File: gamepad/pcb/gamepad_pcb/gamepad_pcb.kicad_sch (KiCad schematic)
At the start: 9 parts, among them J1 RP CON R, J2 RP CON L, J3 JOYSTICK, SW1 BTN MINUS, SW2 BTN PLUS, SW3 BTN NORTH, SW4 BTN EAST, SW5 BTN SOUTH, SW6 BTN WEST

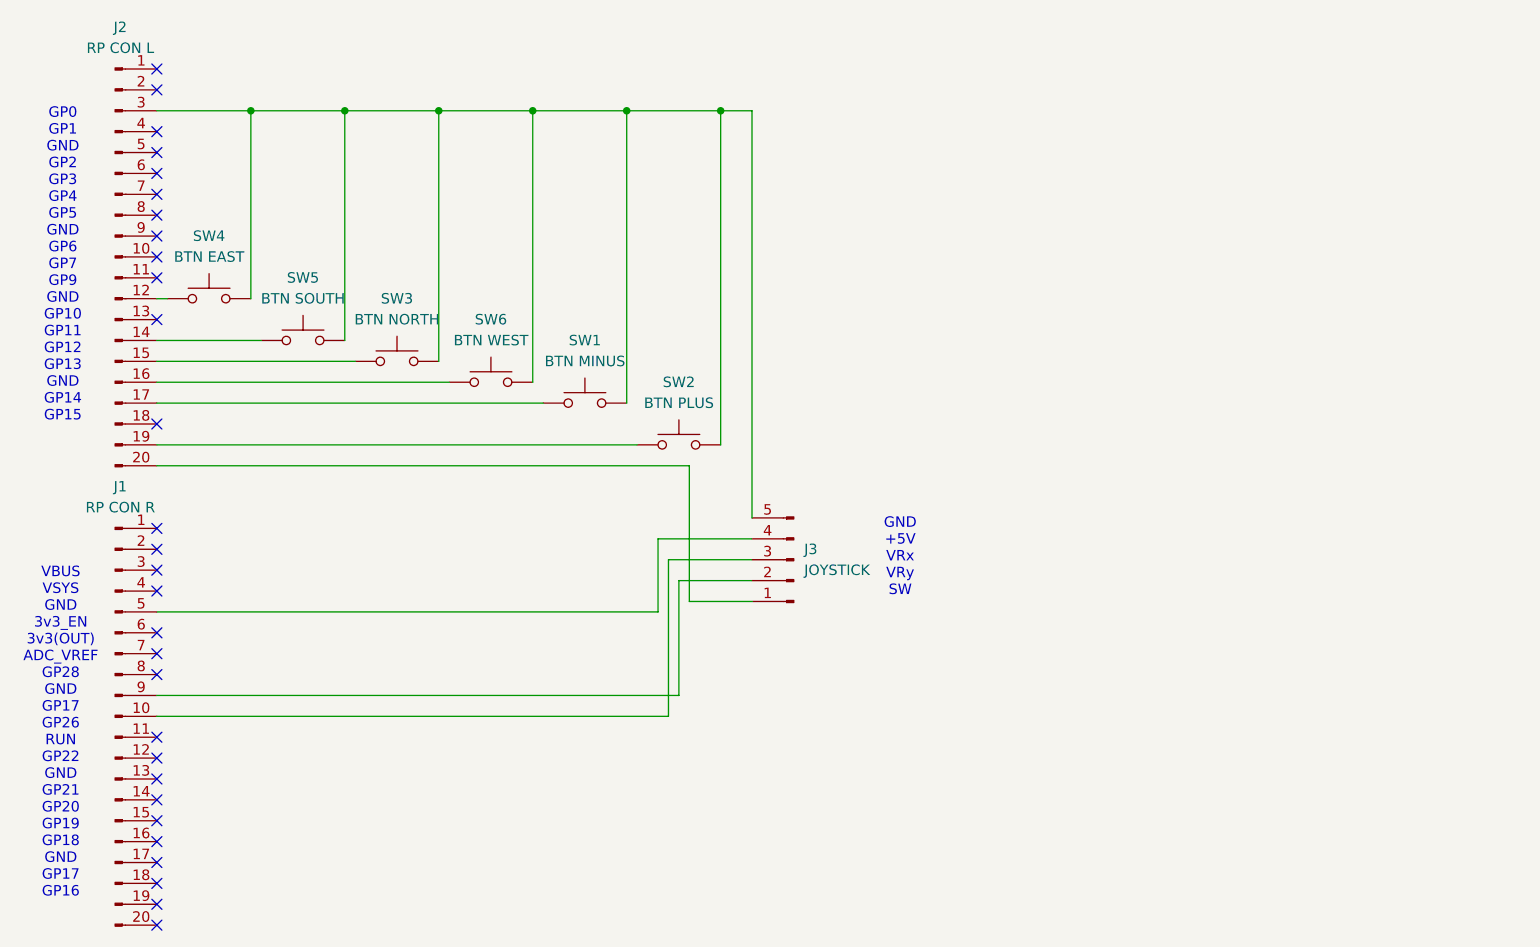
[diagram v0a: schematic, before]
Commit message: feat: working on pcb
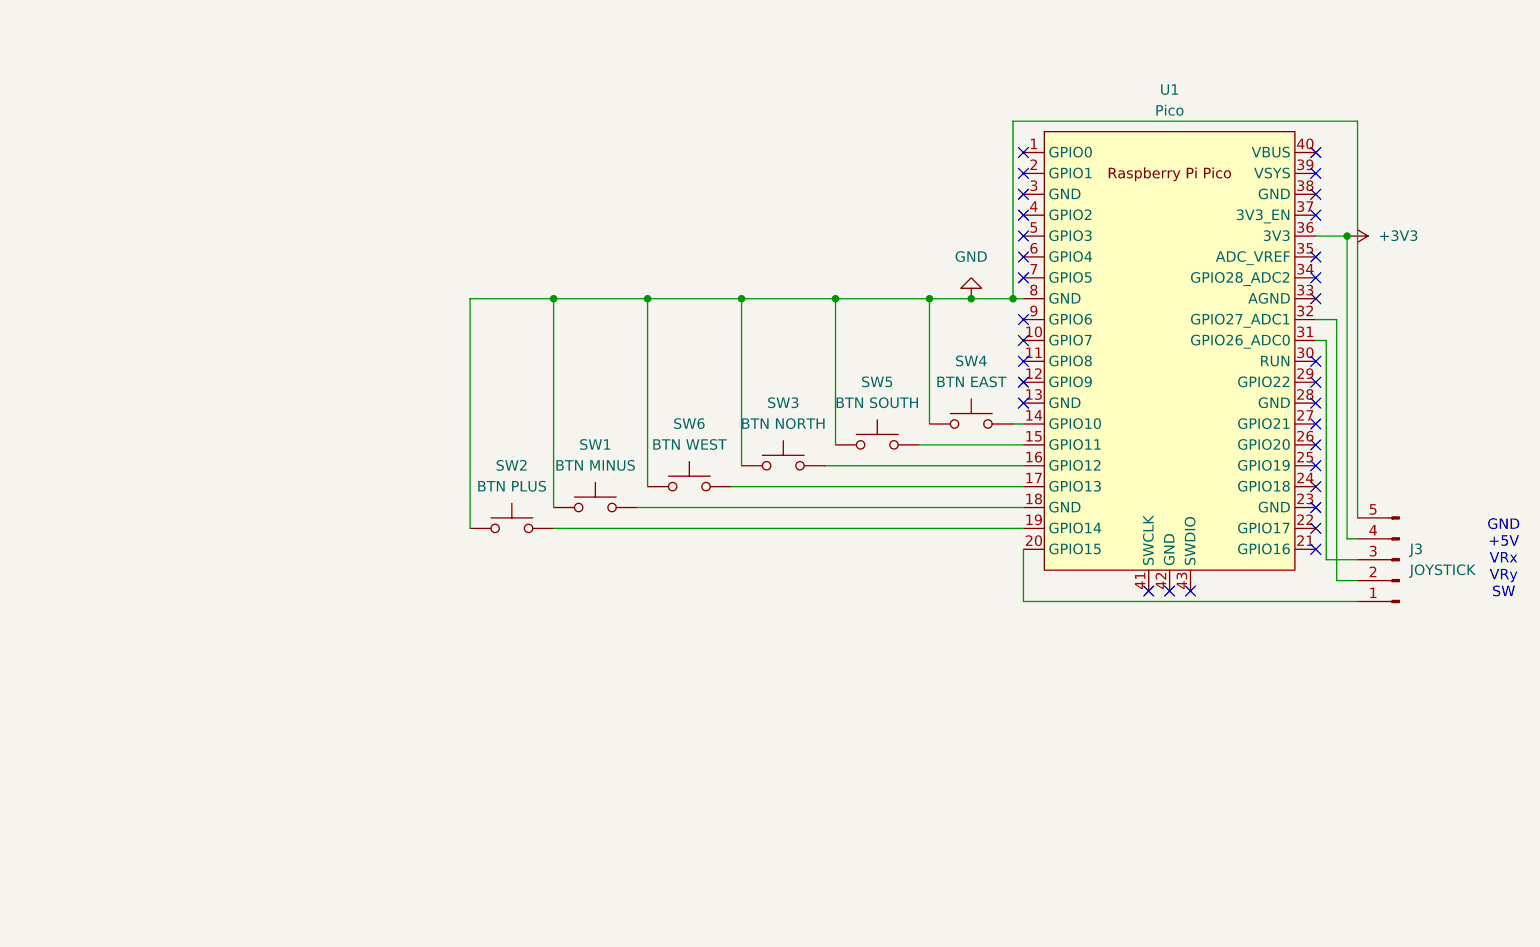
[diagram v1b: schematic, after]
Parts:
- removed J1: RP CON R, Connector_PinSocket_2.54mm:PinSocket_1x20_P2.54mm_Vertical, symbol Connector:Conn_01x20_Pin
- removed J2: RP CON L, Connector_PinSocket_2.54mm:PinSocket_1x20_P2.54mm_Vertical, symbol Connector:Conn_01x20_Pin
- added U1: Pico, RPi_Pico:RPi_Pico_SMD_TH, symbol MCU_RaspberryPi_and_Boards:Pico
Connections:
- net GND: now reaches SW5.1
- net GND: now also J3.5 (Pin_5), SW1.1, SW2.1, SW3.1, SW4.1, SW6.1, U1.8 (GND)
- net at J3.1 (Pin_1): now also U1.20 (GPIO15)
- net at J3.3 (Pin_3): now also U1.31 (GPIO26_ADC0)
- net +3V3: now reaches J3.4 (Pin_4)
- net +3V3: now also U1.36 (3V3)
- net at J3.2 (Pin_2): now also U1.32 (GPIO27_ADC1)
- new net: SW5.2, U1.15 (GPIO11)
- new net: SW4.2, U1.14 (GPIO10)
- new net: SW3.2, U1.16 (GPIO12)
- new net: SW6.2, U1.17 (GPIO13)
- new net: SW1.2, U1.18 (GND)
- new net: SW2.2, U1.19 (GPIO14)
- no-connect marks 29 -> 32
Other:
- note removed: "GP0 GP1 GND GP2 GP3 GP4 GP5 GND GP6 GP7 GP9 GND GP10 GP11 GP12 GP13 GND GP14 GP15"
- note removed: "VBUS VSYS GND 3v3_EN 3v3(OUT) ADC_VREF GP28 GND GP17 GP26 RUN GP22 GND GP21 GP20 GP19 GP18 GND GP17 GP16"
- company: (none) -> ONYX Development
- title: (none) -> Andrew Arcade Controller
- moved on the sheet: J3, SW1, SW2, SW3, SW4, SW5, SW6
